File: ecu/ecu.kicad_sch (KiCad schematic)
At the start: 85 parts, among them J1 INPUTS, J2 OUTPUTS, Q1 AOD4185, Q2 AOD4185, Q3 AOD4185, Q4 BXT3800P06M, Q5 BXT3800P06M, Q6 BXT3800P06M, Q7 BXT3800P06M, Q8 AOD4185, SW1 DISP_BUTTON, U1 MCP2551-I-SN, U2 L6981C33DR, U3 SN65HVD232, U4 ULN2003, U5 ULN2003

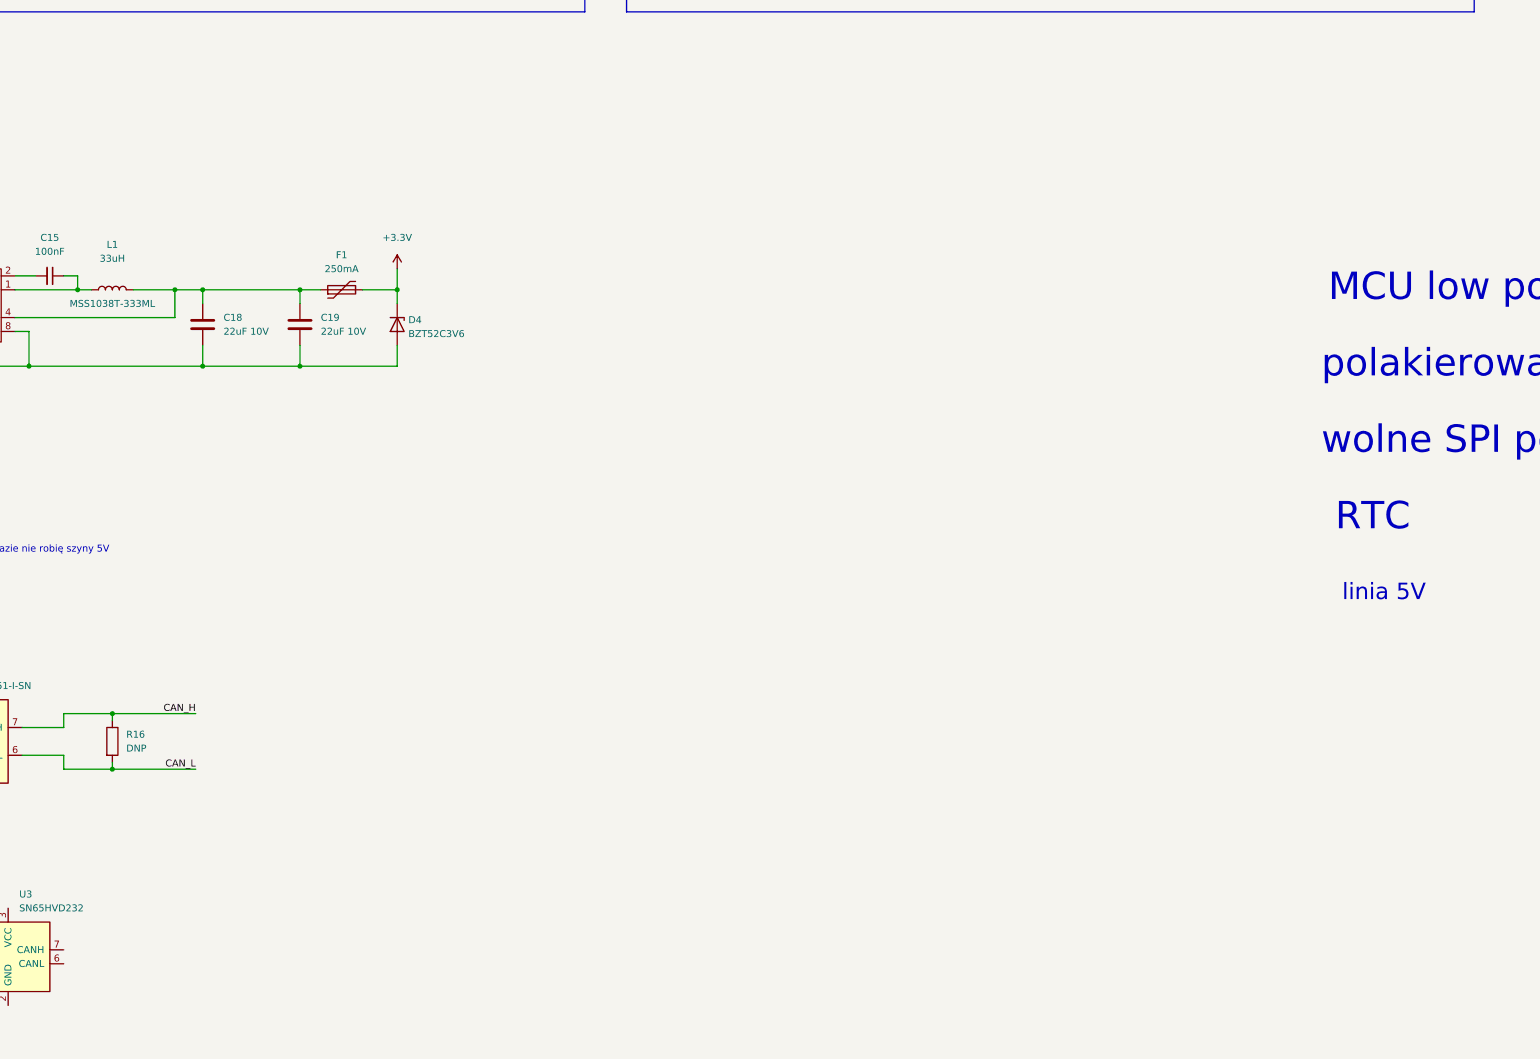
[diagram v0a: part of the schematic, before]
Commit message: stm dodany
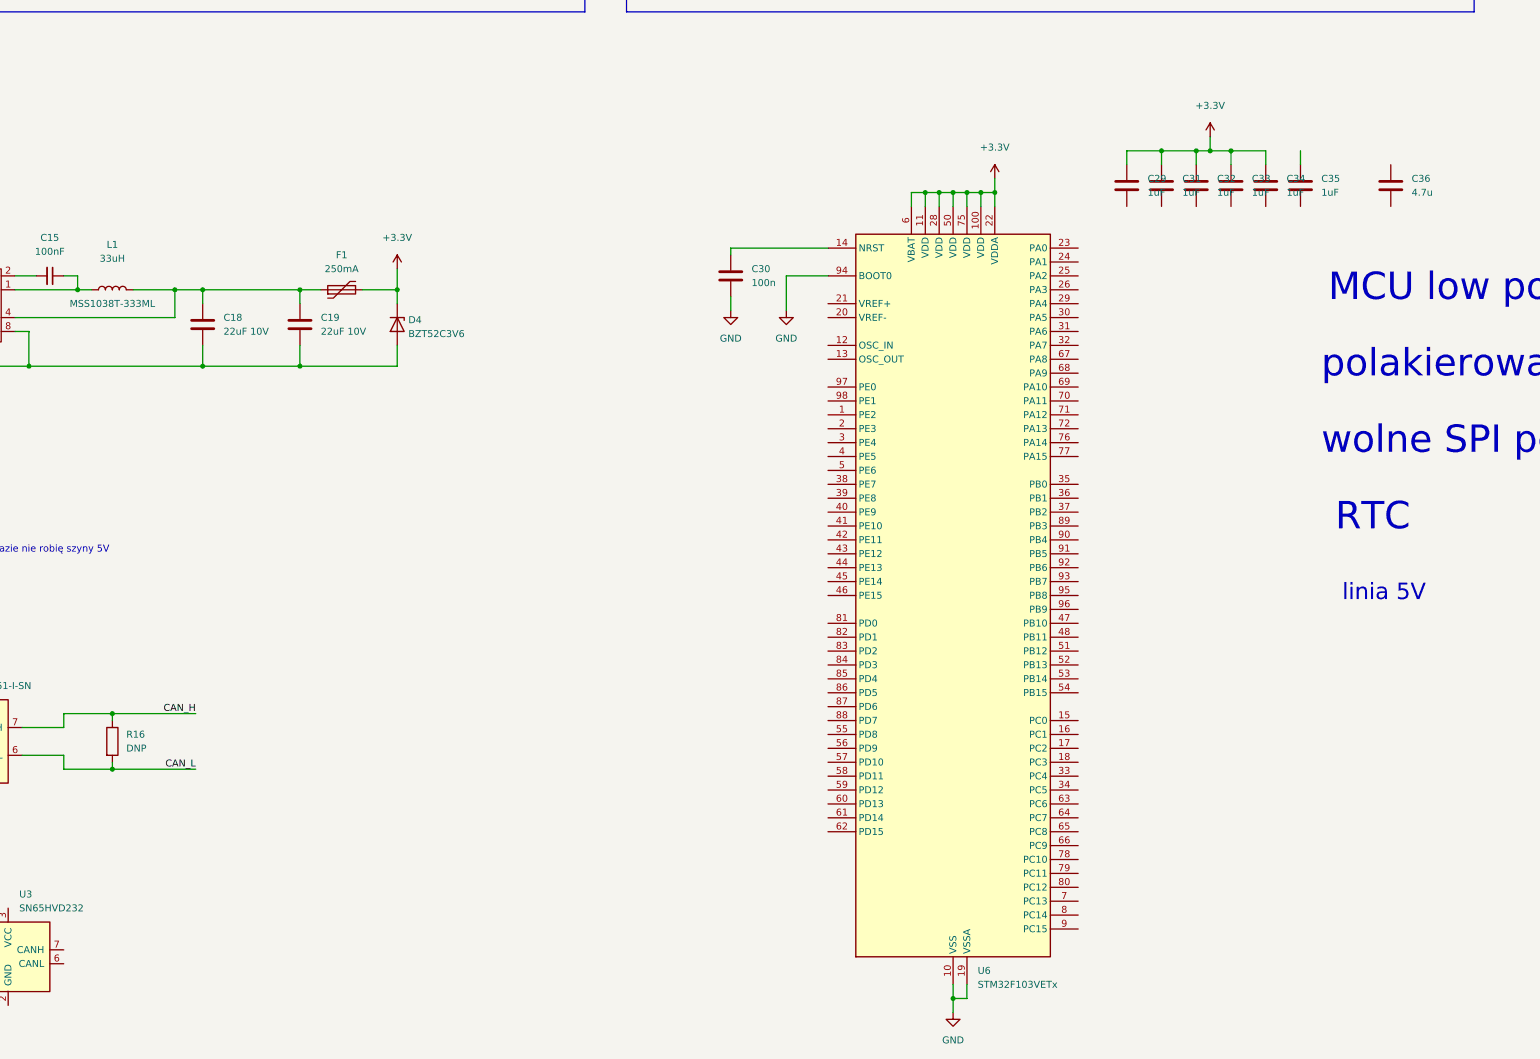
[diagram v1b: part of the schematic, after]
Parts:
- added C29, C31, C32, C33, C34, C35: 1uF, symbol Device:C
- added C30: 100n, symbol Device:C
- added C36: 4.7u, symbol Device:C
- added U6: STM32F103VETx, Package_QFP:LQFP-100_14x14mm_P0.5mm, symbol MCU_ST_STM32F1:STM32F103VETx
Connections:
- net +3V3: now also C29.1, C31.1, C32.1, C33.1, C34.1, U6.100 (VDD), U6.11 (VDD), U6.22 (VDDA), U6.28 (VDD), U6.50 (VDD), U6.6 (VBAT), U6.75 (VDD)
- net GND: now also C30.2, U6.10 (VSS), U6.19 (VSSA), U6.27 (VSS), U6.49 (VSS), U6.74 (VSS), U6.94 (BOOT0), U6.99 (VSS)
- new net: C30.1, U6.14 (NRST)
